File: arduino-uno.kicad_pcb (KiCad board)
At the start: 2 copper layers, 68.6 x 53.3 mm, 52 parts, among them J1 Jack-DC, J2 USB_B, J3 Conn_02x03_Odd_Even, J4 Conn_02x02_Odd_Even, J5 Conn_02x03_Odd_Even, P1 Power, P2 Analog, P3 Digital, P4 Digital, P5 CONN_01X01, P6 CONN_01X01, P7 CONN_01X01, P8 CONN_01X01, Q1 FDN340P, SW1 SW_Push, U1 NCP1117-5.0_SOT223, U2 LMV358IDGKR, U3 LP2985-3.3, U4 ATmega16U2-MU, U5 ATmega328P-PU, Y1 Crystal, Y2 CSTCE16M0V53-R0

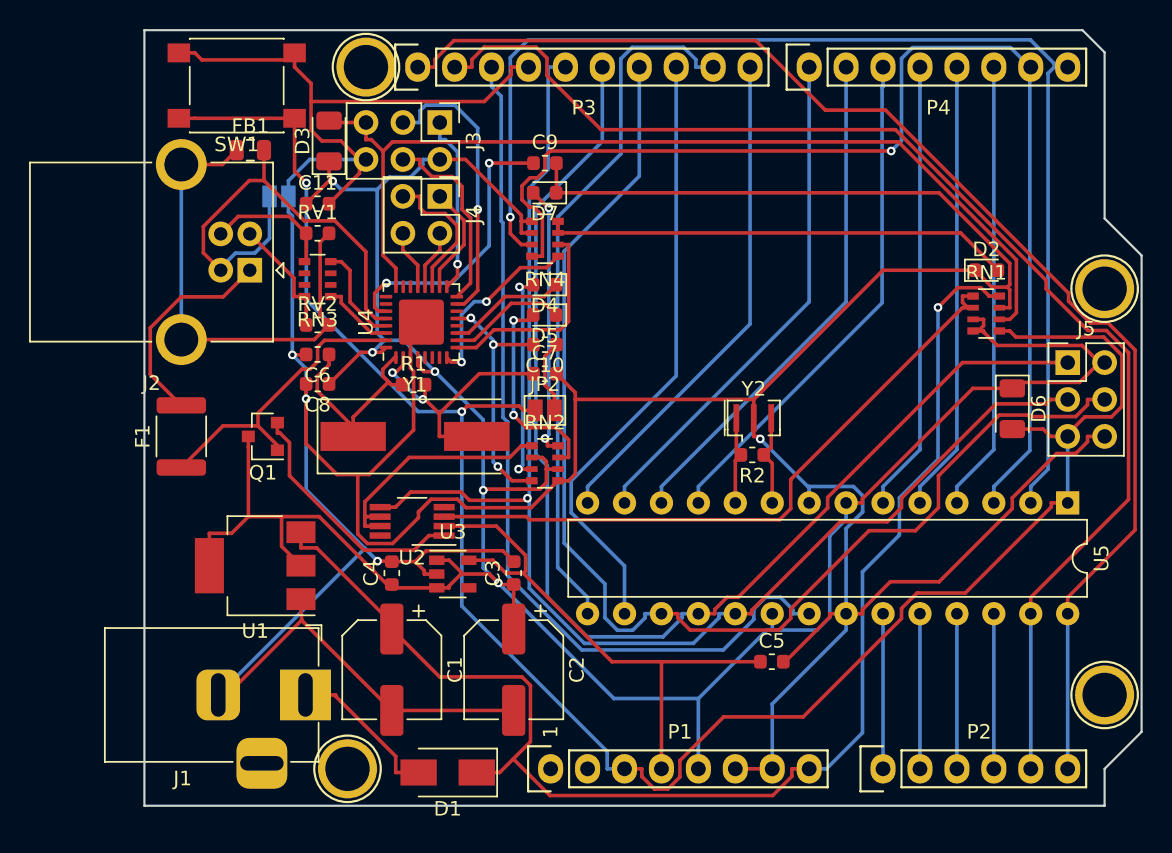
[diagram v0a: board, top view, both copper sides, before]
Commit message: update
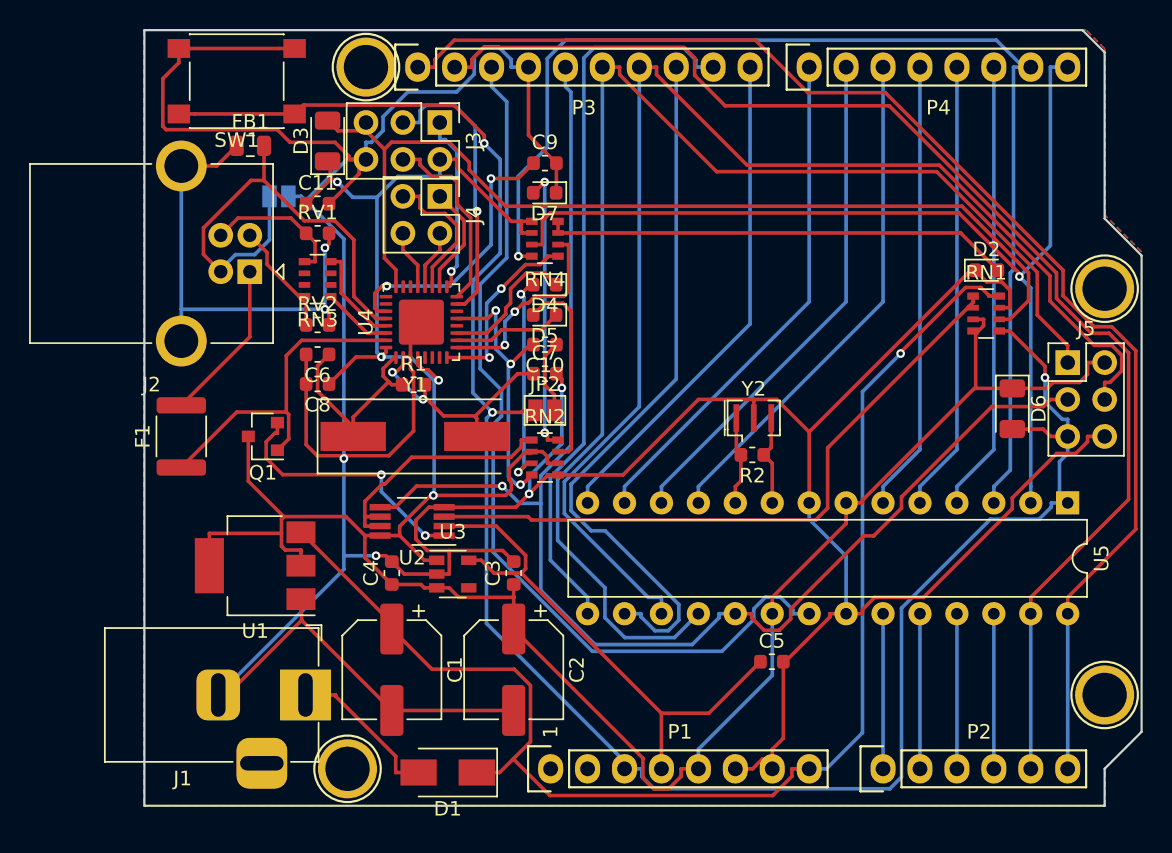
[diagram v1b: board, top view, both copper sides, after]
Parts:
- moved RN2 0.40 mm to (138.5, 102.4)
- moved FB1 0.30 mm to (118.3, 81.0)
- moved SW1 0.30 mm to (117.3, 76.5)
- moved J2 0.10 mm to (118.2, 89.6)
- moved D3 0.10 mm to (123.6, 80.6)
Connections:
- U2 pad 4: (no net) -> GND
- U2 pad 8: (no net) -> +5V
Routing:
- net GND: track 317.2 -> 288.4 mm
- net /Main/0(Rx): track 84.3 -> 69.7 mm
- net /Main/10(**/SS): track 42.1 -> 49.3 mm
- net /Main/12(MISO): track 84.1 -> 91.3 mm
- net /Main/11(**/MOSI): track 85.7 -> 89.5 mm
- net Net-(F1-Pad2): track 14.7 -> 11.1 mm
- net /Main/Reset: track 136.6 -> 139.9 mm, vias 2 -> 3
- net Net-(C7-Pad1): track 18.6 -> 16.0 mm
- net /Power/USBVCC: track 21.0 -> 23.0 mm
- net /Main/9(**): track 48.4 -> 50.3 mm
- net /Main/AREF: track 60.8 -> 62.6 mm
- net /Main/DTR: track 17.5 -> 19.1 mm
- net Net-(D4-Pad1): track 8.21 -> 9.70 mm
- net /Main/13(SCK): track 94.8 -> 96.0 mm
- net +5V: track 186.7 -> 185.7 mm, vias 5 -> 4
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- added copper zone on F.Cu, net GND
- added copper zone on B.Cu, net Net-(FB1-Pad2)
